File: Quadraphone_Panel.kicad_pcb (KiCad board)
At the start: 2 copper layers, 60.8 x 128.5 mm, 31 parts

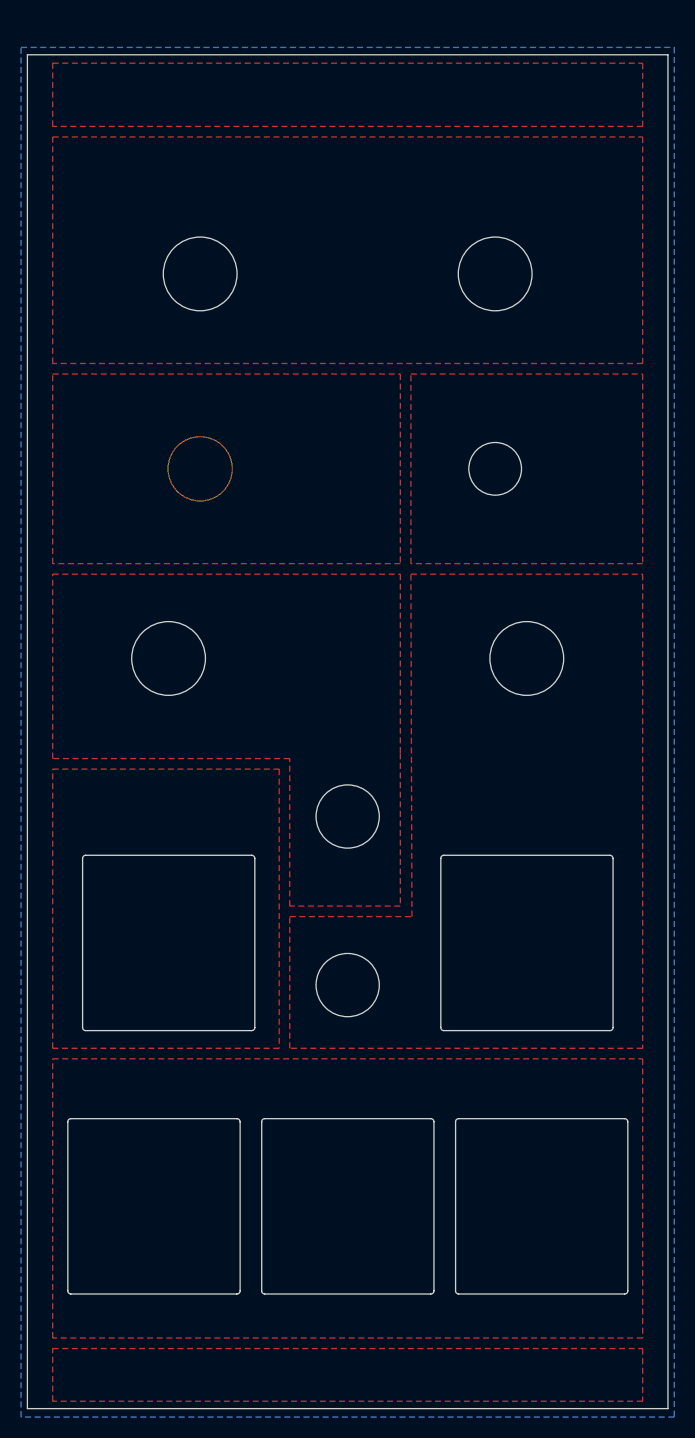
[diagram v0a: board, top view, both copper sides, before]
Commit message: Clean up control board
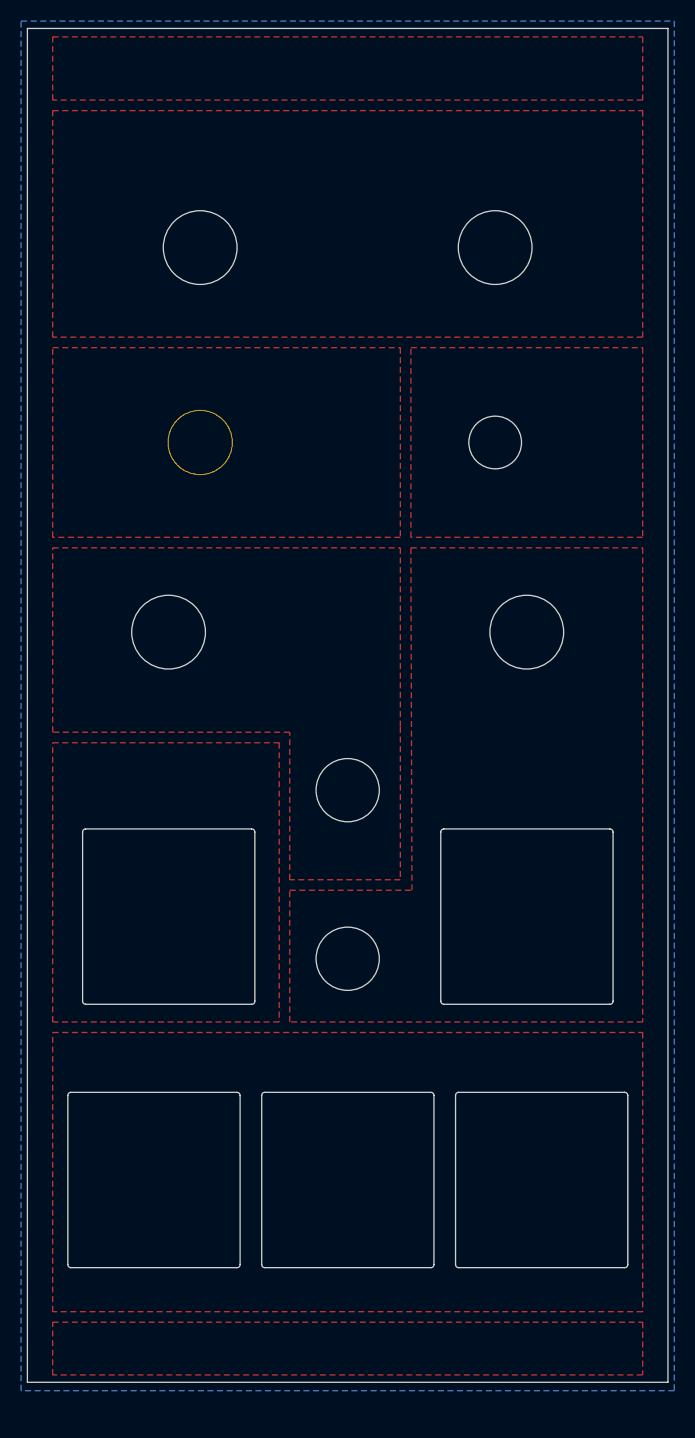
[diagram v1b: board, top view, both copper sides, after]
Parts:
- moved FM_In 2.50 mm to (63.0, 118.5)
- moved G*** 2.50 mm to (80.0, 37.9)
- moved Output 2.50 mm to (80.0, 143.5)
- moved PWM_In 2.50 mm to (97.0, 118.5)
- moved Ref** 2.50 mm to (94.0, 73.5)
- moved Ref** 2.50 mm to (57.1, 159.7)
- moved Ref** 2.50 mm to (80.0, 106.5)
- moved Ref** 2.50 mm to (57.1, 37.2)
- moved Ref** 2.50 mm to (66.0, 55.0)
- moved Ref** 2.50 mm to (102.9, 37.2)
- moved Ref** 2.50 mm to (94.0, 55.0)
- moved Ref** 2.50 mm to (97.0, 91.5)
- moved Ref** 2.50 mm to (66.0, 73.5)
- moved Ref** 2.50 mm to (102.9, 159.7)
- moved Ref** 2.50 mm to (80.0, 122.5)
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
